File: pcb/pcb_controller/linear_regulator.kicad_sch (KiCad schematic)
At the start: 24 parts, among them IC301 OPA277, IC302 OPA277, Q304 BC557

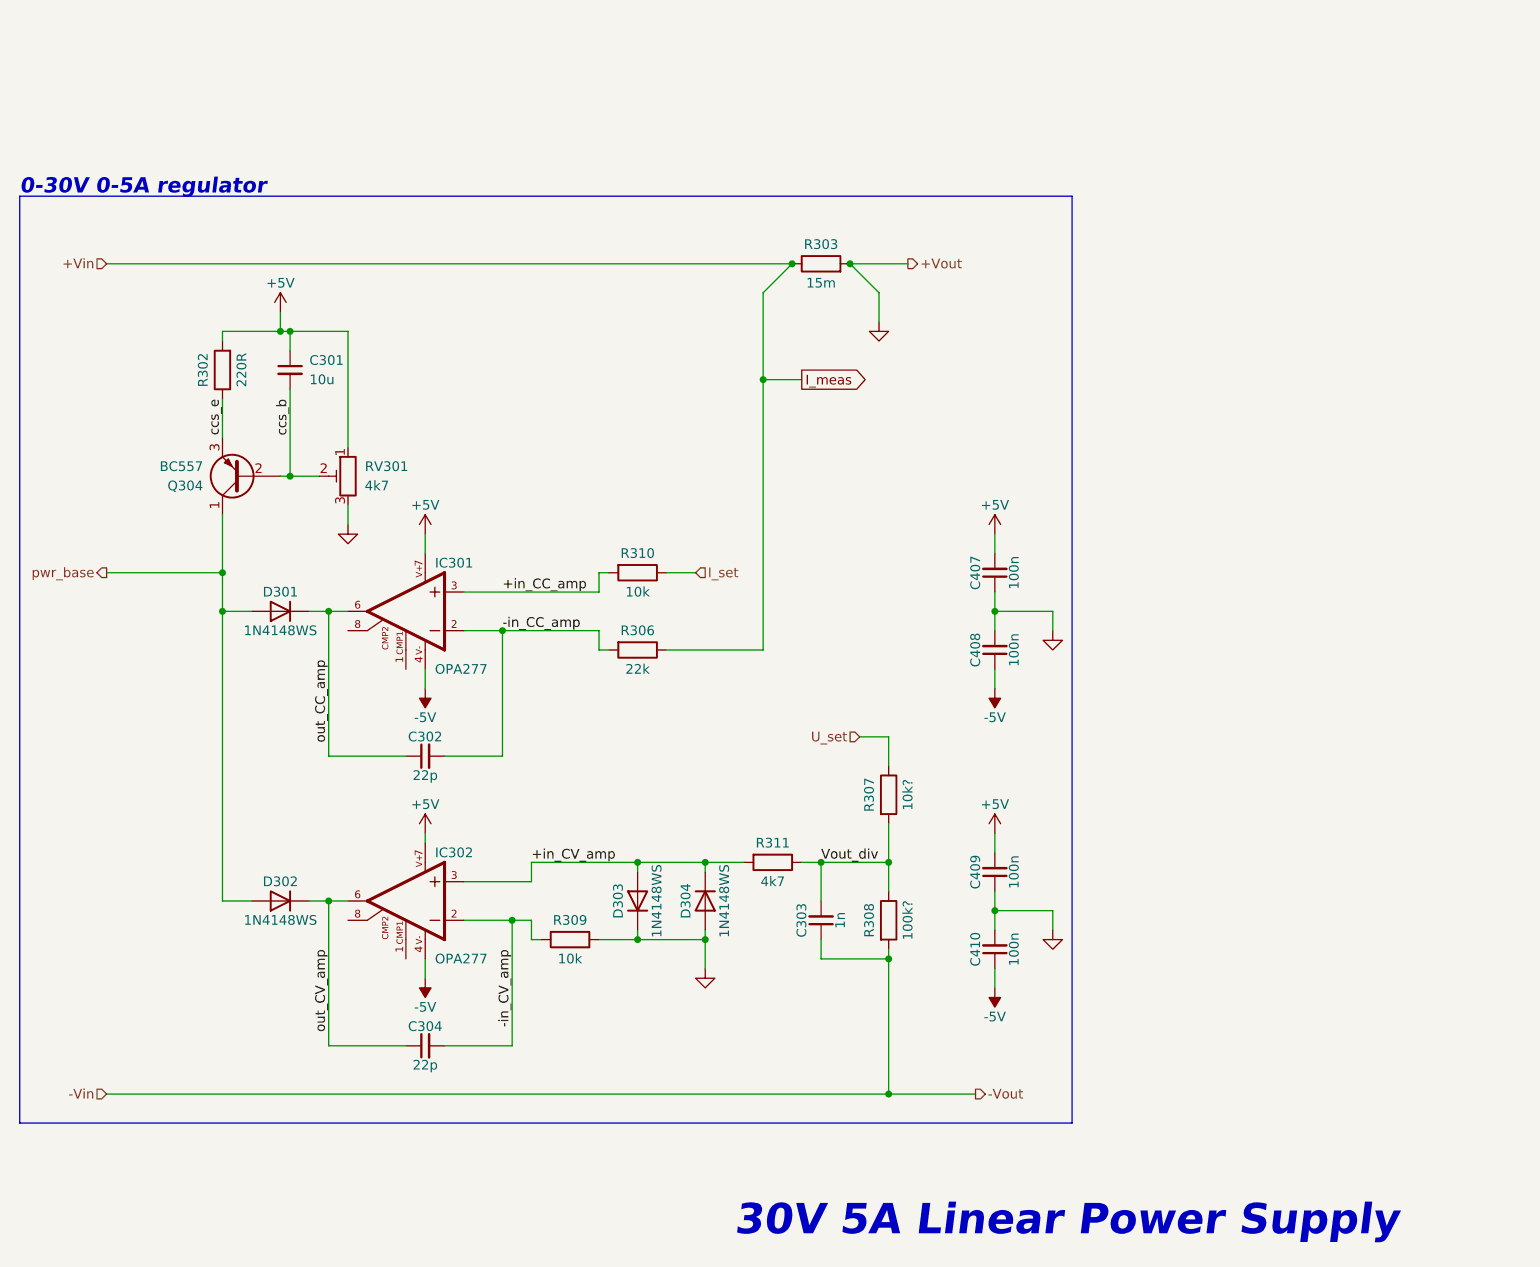
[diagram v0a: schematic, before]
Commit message: most analog layout
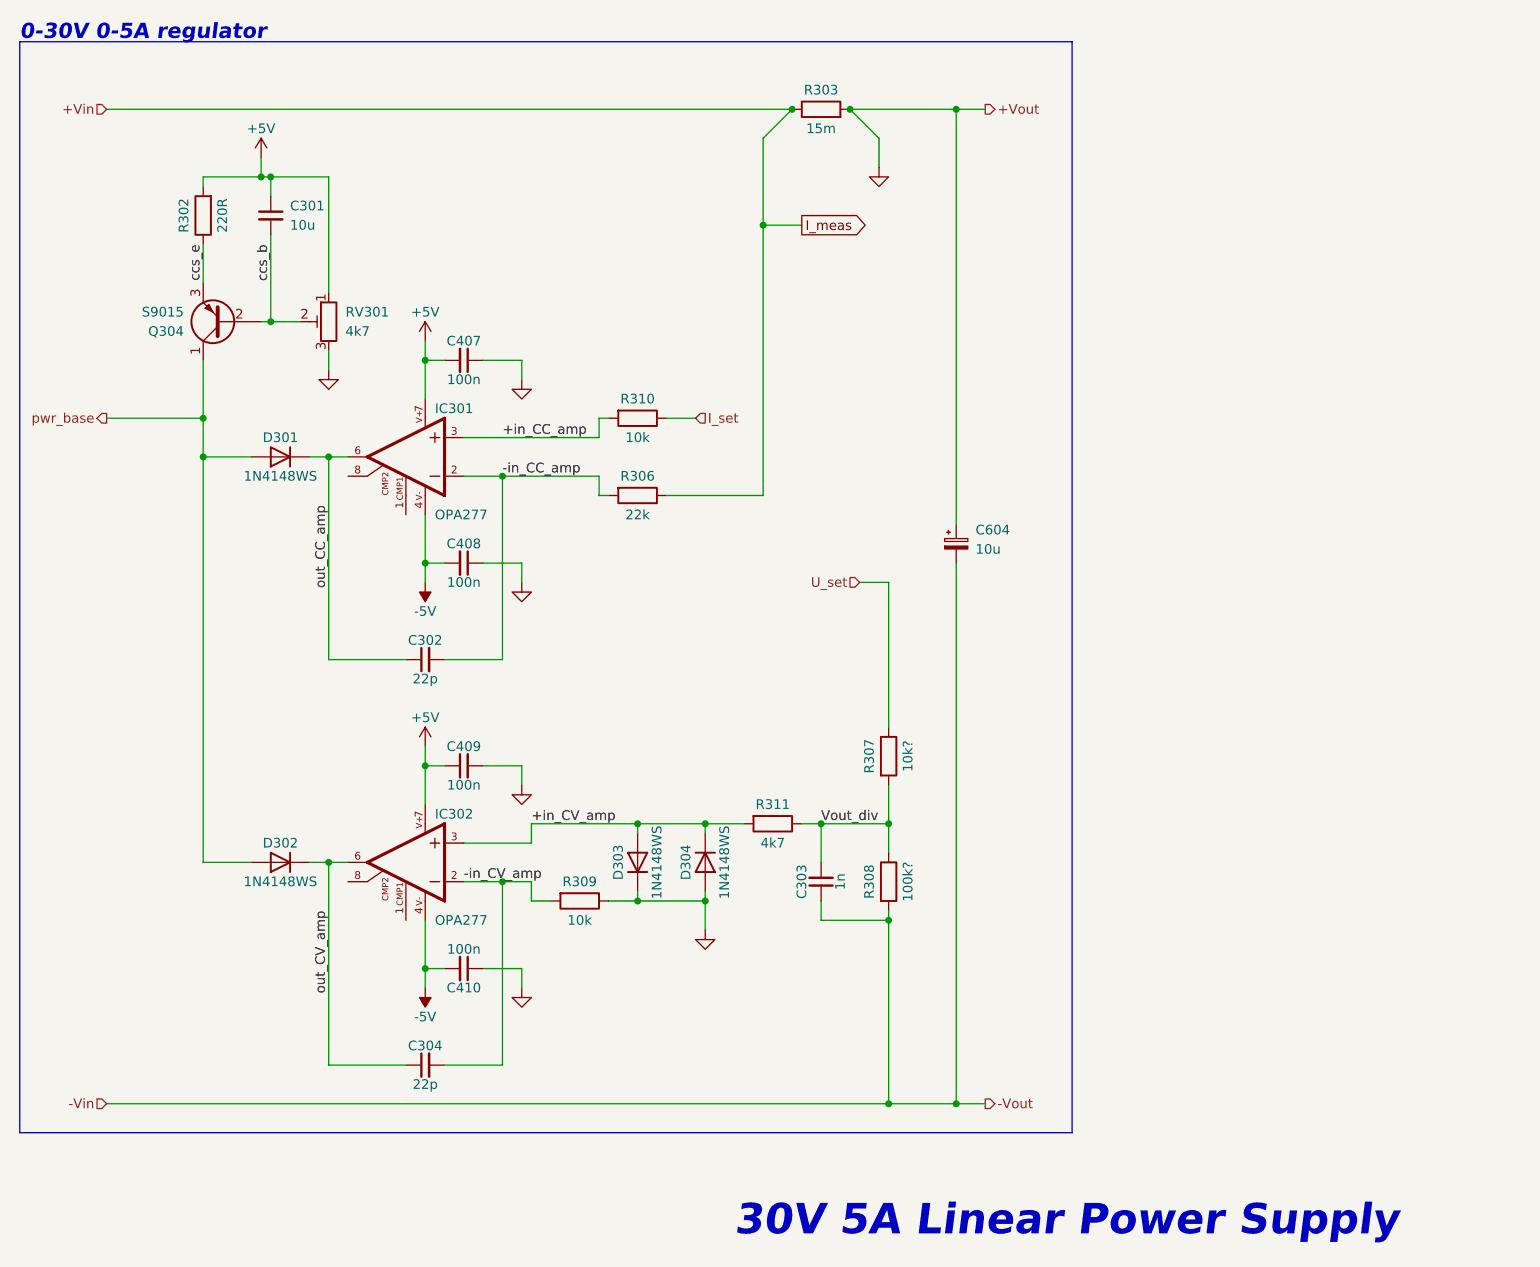
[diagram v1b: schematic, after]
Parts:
- added C604: 10u, Capacitor_THT:CP_Radial_D5.0mm_P2.00mm, symbol Device:C_Polarized_Small
- Q304: value BC557 -> S9015
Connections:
- net +5V: now also C409.1; no longer C409.2
- net -5V: now also C408.2, C410.2; no longer C408.1, C410.1
- net -Vin: now also C604.2
- net GND: now also C408.1, C409.2, C410.1, C604.1; no longer C408.2, C409.1, C410.2
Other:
- moved on the sheet: C301, C302, C303, C304, C407, C408, C409, C410, D301, D302, D303, D304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
